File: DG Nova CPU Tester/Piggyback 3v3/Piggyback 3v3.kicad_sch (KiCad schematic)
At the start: 22 parts, among them J10 Programmed I/O, J11 CPU Option Inputs, J12 Data Channel, J13 Program Interrupt, J14 System Control, J17 CPU Option Outputs, J18 MEM Control Outputs, J19 Logic 8 CH, J20 Logic 8 CH, J6 MBO, J7 MEM, J8 Data Channel, J9 Front Panel Controls, U1 74LS125, U2 Pico, U25 74AHC244, U26 74HCT244

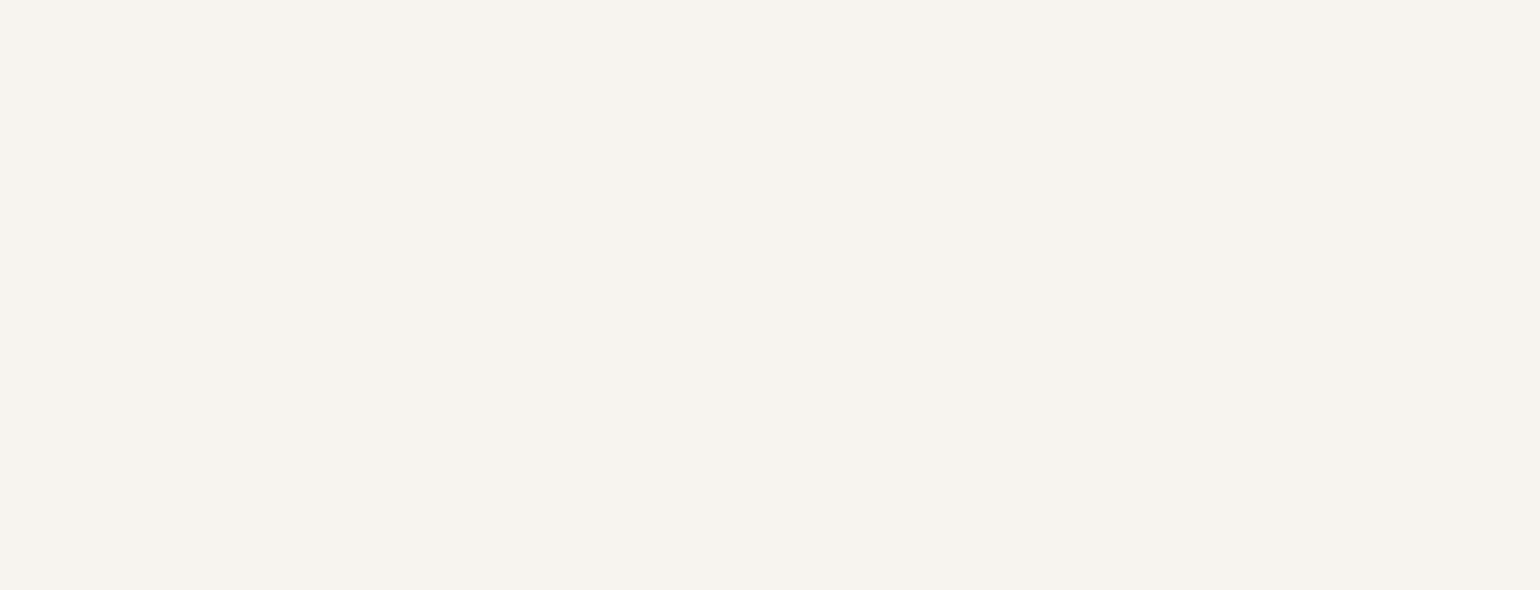
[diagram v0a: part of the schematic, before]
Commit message: GPIO research
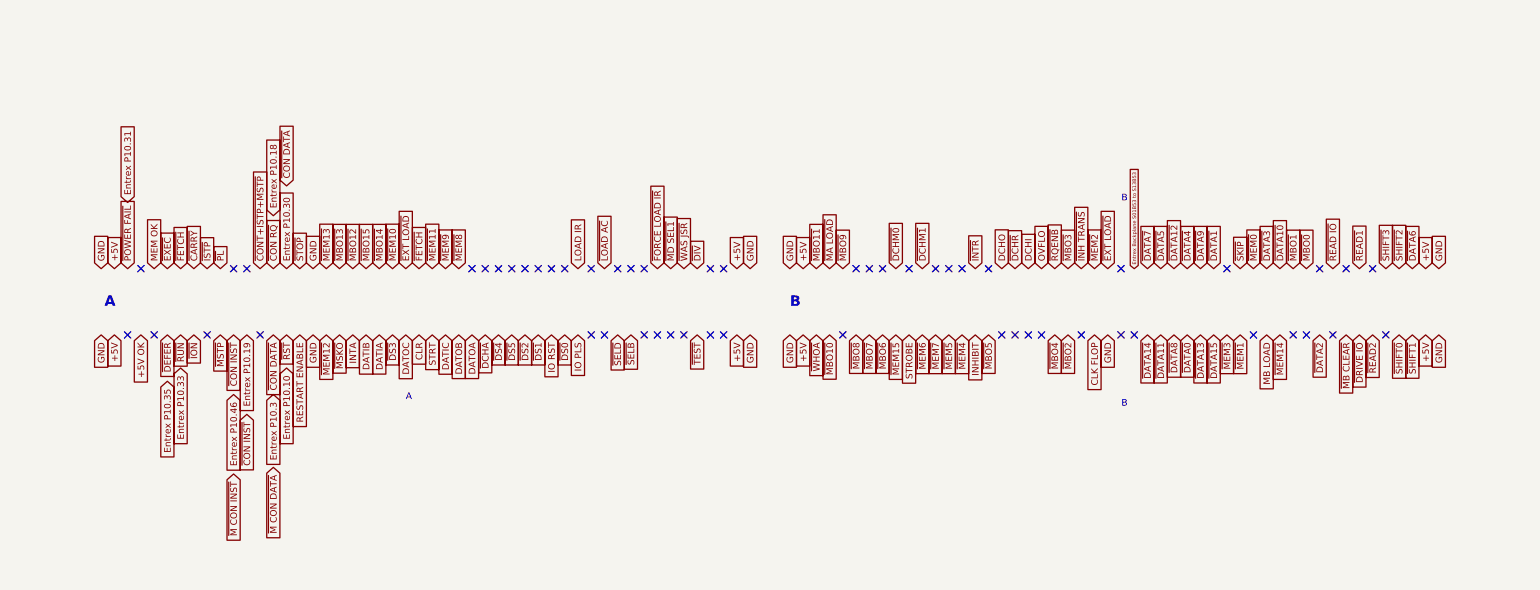
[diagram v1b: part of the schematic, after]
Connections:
- no-connect marks 0 -> 55
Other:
- note added: "A"
- note added: "B"
